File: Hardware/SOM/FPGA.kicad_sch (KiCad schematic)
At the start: 46 parts, among them U1 LFE5UM5G-85F

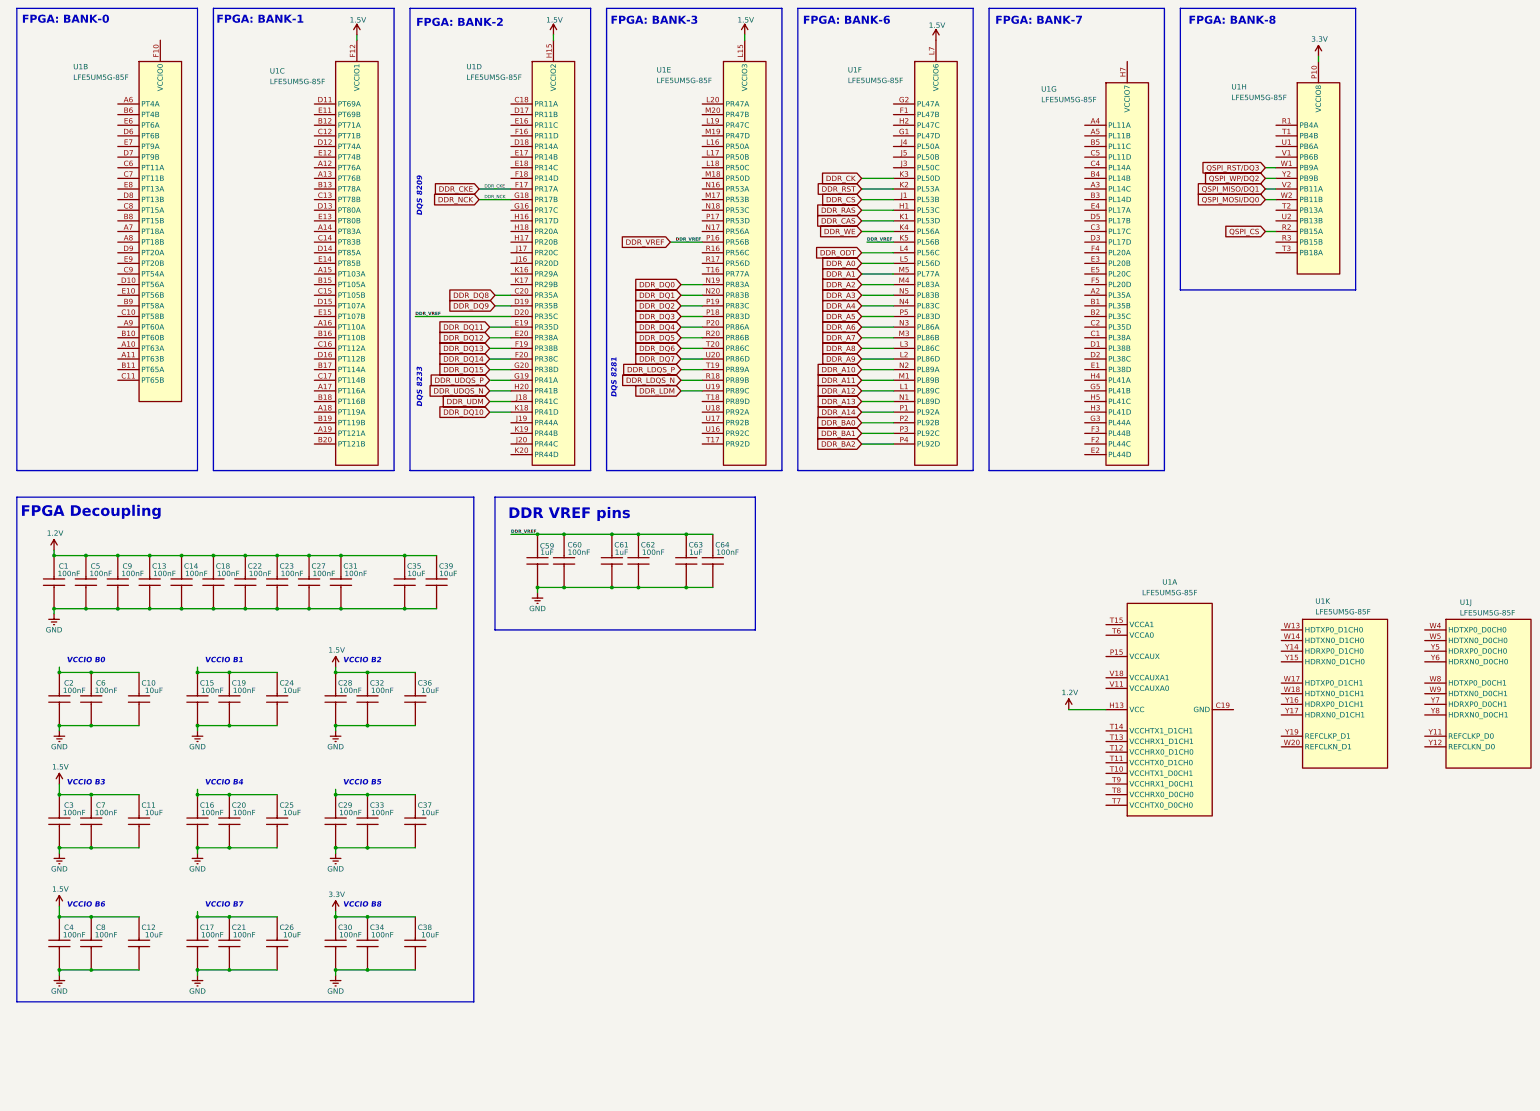
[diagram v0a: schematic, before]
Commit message: SOM: power supplies
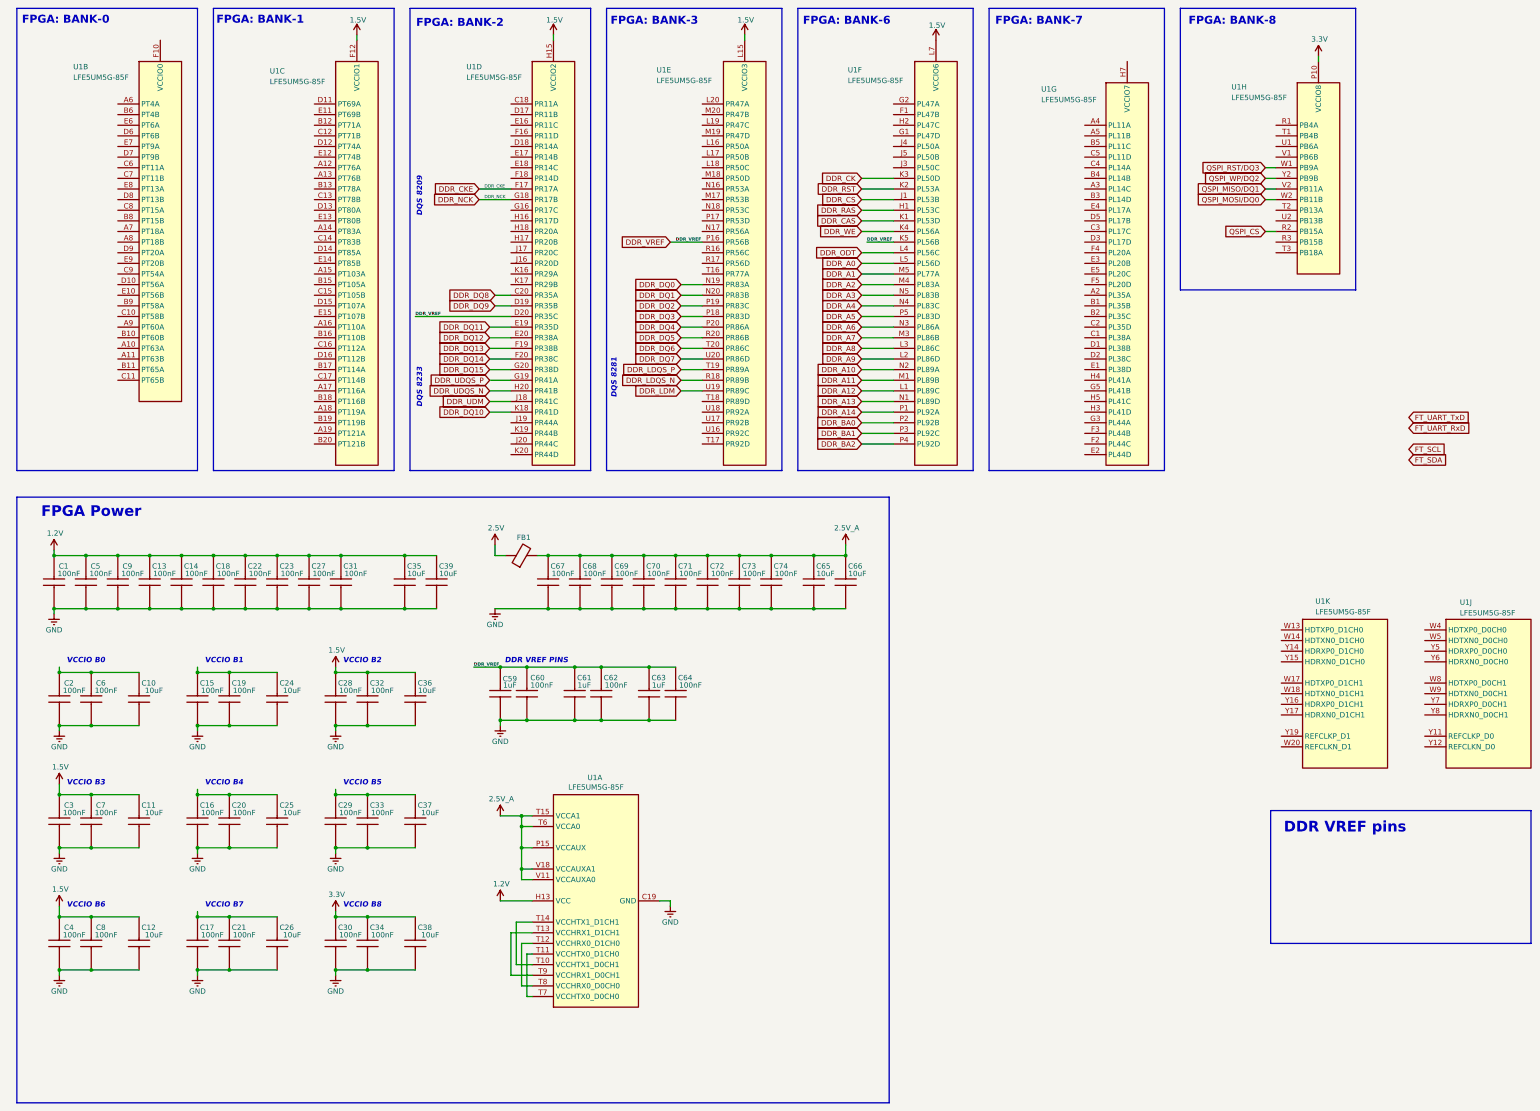
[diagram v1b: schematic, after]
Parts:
- added C65, C66: 10uF, Capacitor_SMD:C_0402_1005Metric, symbol RA8M1:885012205092
- added C67, C68, C69, C70, C71, C72, C73, C74: 100nF, Capacitor_SMD:C_0402_1005Metric, symbol RA8M1:885012205092
- added FB1: FerriteBead, Inductor_SMD:L_1206_3216Metric, symbol Device:FerriteBead
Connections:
- net GND: now also U1.B14 (GND), U1.B7 (GND), U1.C19 (GND), U1.D4 (GND), U1.F13 (GND), U1.F14 (GND), U1.F7 (GND), U1.F8 (GND), U1.G10 (GND), U1.G11 (GND), U1.G12 (GND), U1.G13 (GND), U1.G14 (GND), U1.G15 (GND), U1.G17 (GND), U1.G4 (GND), U1.G6 (GND), U1.G7 (GND), U1.G8 (GND), U1.G9 (GND), U1.H19 (GND), U1.J10 (GND), U1.J11 (GND), U1.J12 (GND), U1.J14 (GND), U1.J2 (GND), U1.J7 (GND), U1.J9 (GND), U1.K10 (GND), U1.K11 (GND), U1.K12 (GND), U1.K14 (GND), U1.K15 (GND), U1.K6 (GND), U1.K7 (GND), U1.K9 (GND), U1.L10 (GND), U1.L11 (GND), U1.L12 (GND), U1.L9 (GND), U1.M10 (GND), U1.M11 (GND), U1.M12 (GND), U1.M14 (GND), U1.M16 (GND), U1.M2 (GND), U1.M7 (GND), U1.M9 (GND), U1.N14 (GND), U1.N15 (GND), U1.N6 (GND), U1.N7 (GND), U1.P11 (GND), U1.P12 (GND), U1.P13 (GND), U1.P14 (GND), U1.P7 (GND), U1.P8 (GND), U1.R19 (GND), U1.U10 (GND), U1.U11 (GND), U1.U12 (GND), U1.U13 (GND), U1.U14 (GND), U1.U7 (GND), U1.U8 (GND), U1.U9 (GND), U1.V12 (GND), U1.V13 (GND), U1.V14 (GND), U1.V15 (GND), U1.V16 (GND), U1.V19 (GND), U1.V20 (GND), U1.V5 (GND), U1.V6 (GND), U1.V7 (GND), U1.V8 (GND), U1.V9 (GND), U1.W12 (GND), U1.W15 (GND), U1.W16 (GND), U1.W19 (GND), U1.W6 (GND), U1.W7 (GND), C65.1, C66.1, C67.1, C68.1, C69.1, C70.1, C71.1, C72.1, C73.1, C74.1
- net 2.5V_A: now reaches U1.F15 (VCCAUX), U1.F6 (VCCAUX), U1.P15 (VCCAUX), U1.P6 (VCCAUX)
- net 2.5V_A: now also U1.T15 (VCCA1), U1.T6 (VCCA0), U1.U15 (VCCA1), U1.U6 (VCCA0), U1.V10 (VCCAUXA0), U1.V11 (VCCAUXA0), U1.V17 (VCCAUXA1), U1.V18 (VCCAUXA1), C65.2, C66.2, C67.2, C68.2, C69.2, C70.2, C71.2, C72.2, C73.2, C74.2, FB1.2
- net at U1.T10 (VCCHTX1_D0CH1): now also U1.T14 (VCCHTX1_D1CH1)
- net at U1.T11 (VCCHTX0_D1CH0): now also U1.T7 (VCCHTX0_D0CH0)
- net at U1.T12 (VCCHRX0_D1CH0): now also U1.T8 (VCCHRX0_D0CH0)
- net at U1.T13 (VCCHRX1_D1CH1): now also U1.T9 (VCCHRX1_D0CH1)
- new net 2.5V: FB1.1
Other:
- note added: "DDR VREF PINS"
- note added: "FPGA Power"
- note removed: "FPGA Decoupling"
- moved on the sheet: C59, C60, C61, C62, C63, C64, U1A
